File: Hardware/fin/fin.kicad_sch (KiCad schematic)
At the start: 39 parts, among them J1 Conn_01x10_Pin, J2 Conn_01x04_Pin, J3 Conn_01x04_Pin, J5 Conn_01x04_Pin, U1 ADS131M03QPWRQ1, U2 STM32L412C8Tx, U3 W25N512GVEIG, U4 TMP235A4DBZR, U5 STM32L412K8Ux

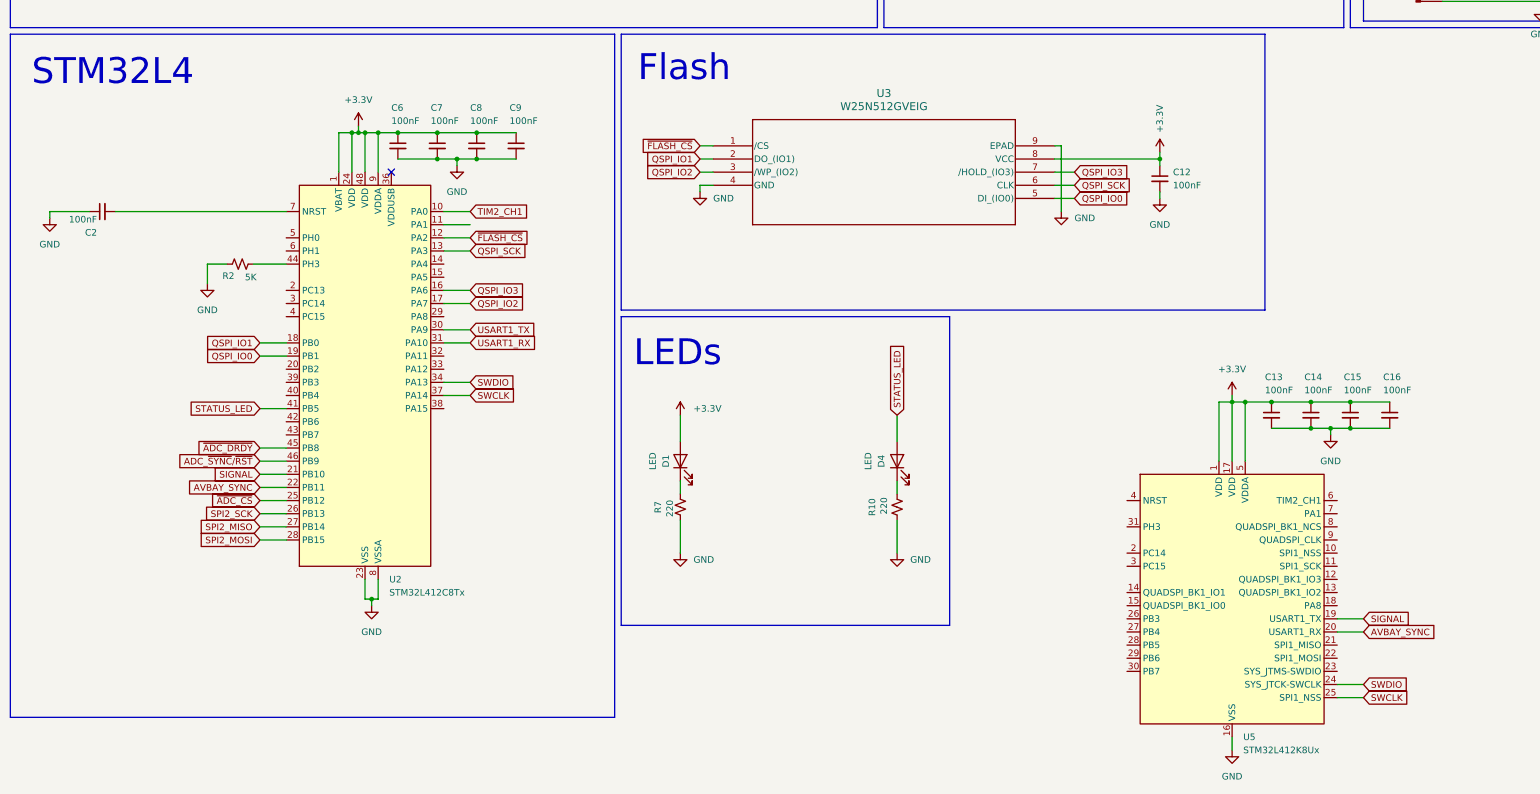
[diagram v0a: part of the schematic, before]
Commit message: updated fin schem
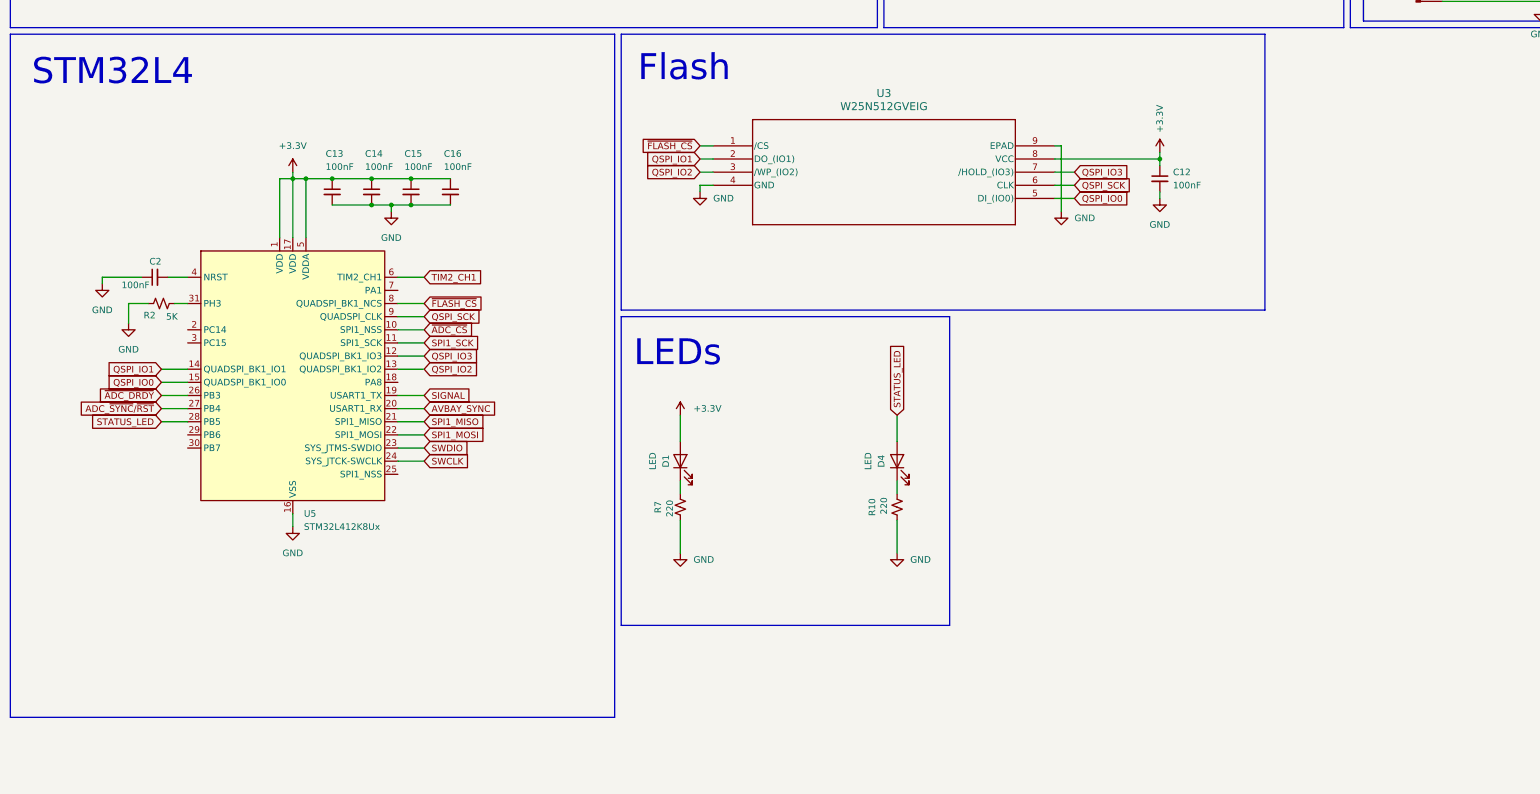
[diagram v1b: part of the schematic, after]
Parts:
- removed C6, C7, C8, C9: 100nF, Capacitor_SMD:C_0603_1608Metric, symbol Device:C_Small
- removed U2: STM32L412C8Tx, Package_QFP:LQFP-48_7x7mm_P0.5mm, symbol MCU_ST_STM32L4:STM32L412C8Tx
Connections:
- net ADC_~{SYNC}/~{RST}: now also U5.27 (PB4)
- net QSPI_IO0: now also U5.15 (PB1)
- net QSPI_IO1: now also U5.14 (PB0)
- net QSPI_IO2: now also U5.13 (PA7)
- net QSPI_IO3: now also U5.12 (PA6)
- net QSPI_SCK: now also U5.9 (PA3)
- net STATUS_LED: now also U5.28 (PB5)
- net SWCLK: now also U5.24 (PA14); no longer U5.25 (PA15)
- net SWDIO: now also U5.23 (PA13); no longer U5.24 (PA14)
- net TIM2_CH1: now also U5.6 (PA0)
- net ~{ADC_CS}: now also U5.10 (PA4)
- net ~{ADC_DRDY}: now also U5.26 (PB3)
- net ~{FLASH_CS}: now also U5.8 (PA2)
- net SPI1_SCK: now reaches U5.11 (PA5)
- net SPI1_MISO: now reaches U5.21 (PA11)
- net SPI1_MOSI: now reaches U5.22 (PA12)
- net at U5.31 (PH3): now also R2.2
- net at U5.4 (NRST): now also C2.2
- no-connect marks 1 -> 0
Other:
- moved on the sheet: C13, C14, C15, C16, C2, R2, U5
